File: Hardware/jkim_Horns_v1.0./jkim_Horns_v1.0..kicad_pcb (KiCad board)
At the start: 2 copper layers, 21 parts, among them J1 Conn_01x03, J2 Conn_01x02, J3 Conn_01x02, J4 Conn_01x02, Q1 Q_NMOS_DGS

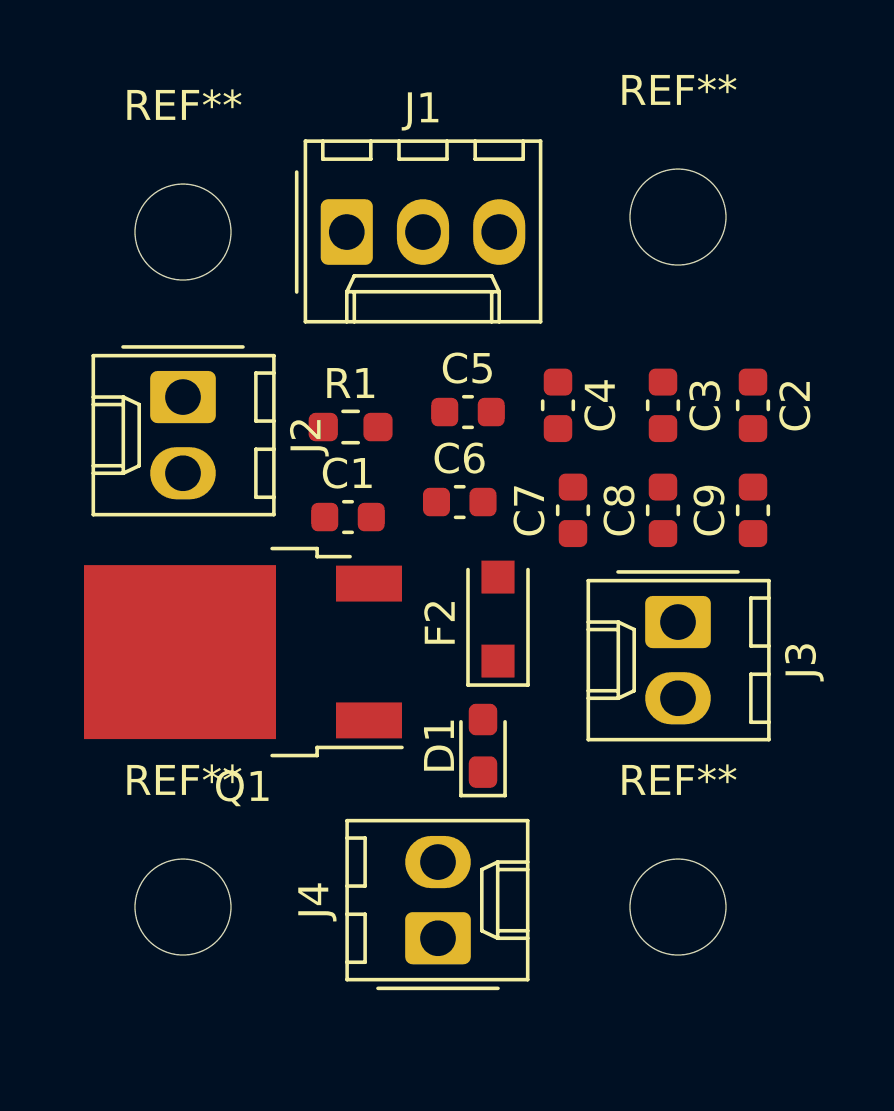
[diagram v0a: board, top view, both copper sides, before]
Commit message: Finished layout
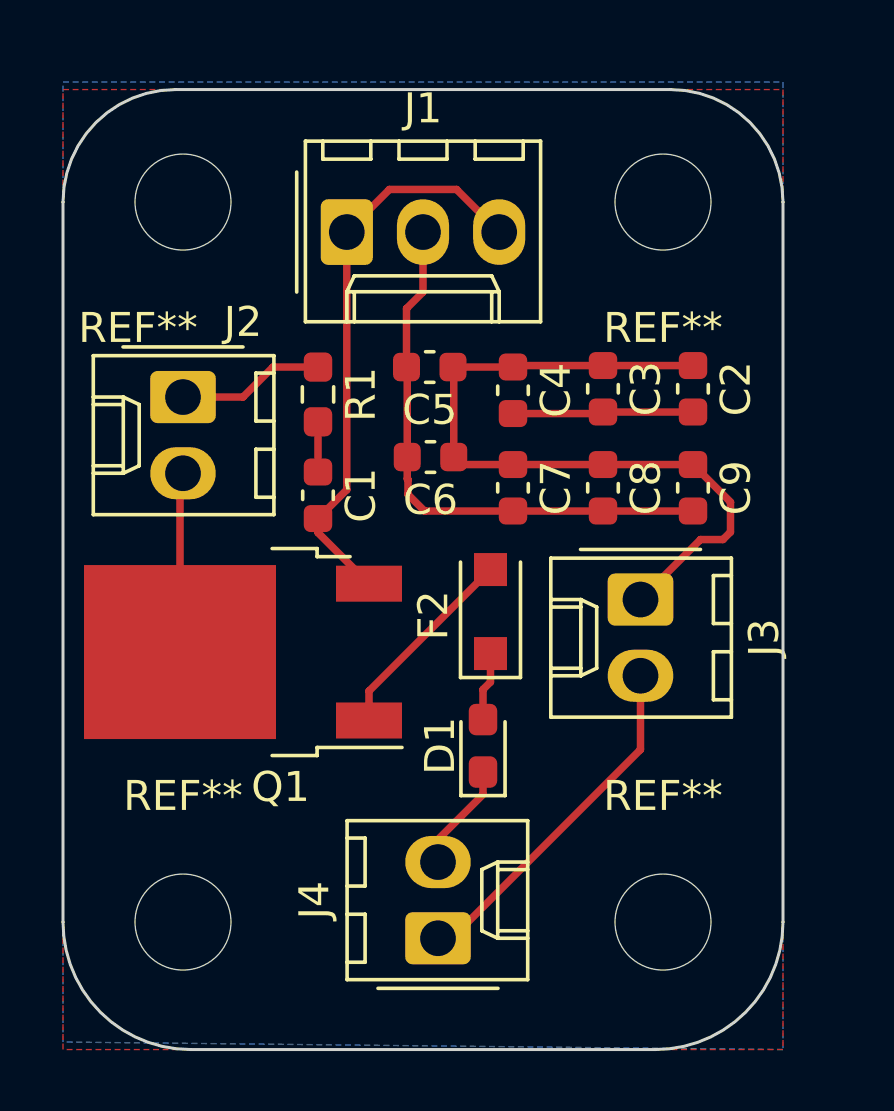
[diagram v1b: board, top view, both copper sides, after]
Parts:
- moved C7 2.14 mm to (67.0, 72.0), turned to -90 degrees
- moved C8 2.14 mm to (70.0, 72.0), turned to -90 degrees
- moved C9 2.14 mm to (73.0, 72.0), turned to -90 degrees
- moved C2 2.07 mm to (73.0, 68.7)
- moved C3 2.07 mm to (70.0, 68.7)
- moved C5 1.97 mm to (64.2, 68.0), turned to 180 degrees
- moved C6 1.79 mm to (64.2, 71.0), turned to 180 degrees
- moved C4 1.58 mm to (67.0, 68.8)
- moved R1 1.54 mm to (60.5, 68.9), turned to -90 degrees
- moved J3 1.46 mm to (71.2, 75.8)
- moved C1 1.24 mm to (60.5, 72.3), turned to -90 degrees
- moved REF** 1.00 mm to (56.0, 62.5), turned to 180 degrees
- moved REF** 0.71 mm to (72.0, 86.5)
- moved REF** 0.71 mm to (72.0, 62.5), turned to 180 degrees
- moved REF** 0.50 mm to (56.0, 86.5)
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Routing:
- net Net-(J3-Pin_1): track 0.00 -> 25.8 mm
- net +24V: track 0.00 -> 24.7 mm
- net GND: track 0.00 -> 19.2 mm
- net Net-(J3-Pin_2): track 0.00 -> 12.1 mm
- net Net-(Q1-D): track 0.00 -> 6.71 mm
- net /HORN_CTL: track 0.00 -> 6.00 mm
- net Net-(J2-Pin_1): track 0.00 -> 4.91 mm
- net Net-(D1-K): track 0.00 -> 3.62 mm
- net /HORN_IN: track 0.00 -> 2.30 mm
- net Net-(C1-Pad1): track 0.00 -> 1.67 mm
- added copper zone on F.Cu, net +24V
- added copper zone on B.Cu, net GND
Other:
- board outline added: 24 x 32 mm
